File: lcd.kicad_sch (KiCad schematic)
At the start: 4 parts, among them J5 LS013B7DH03

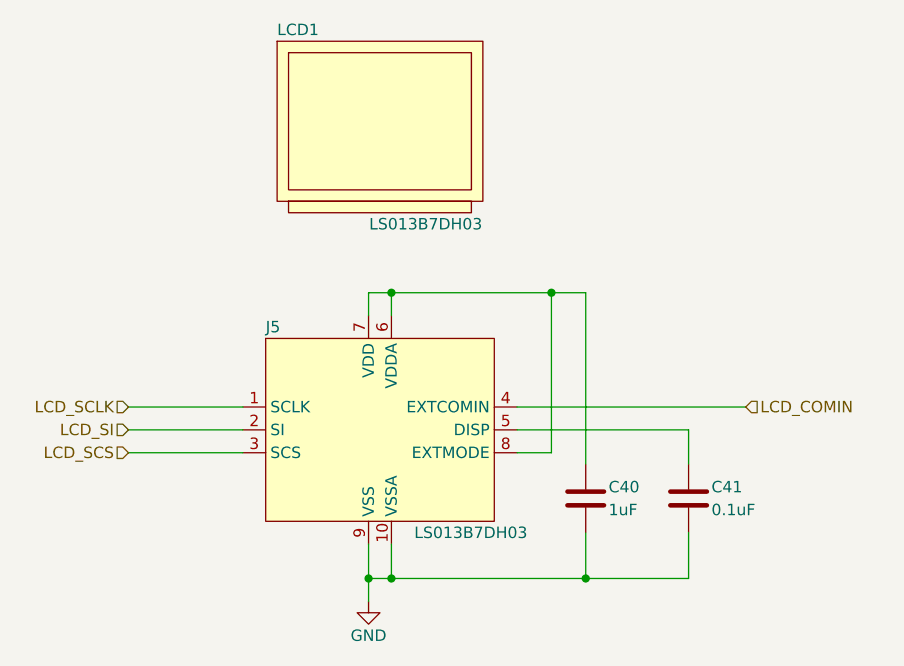
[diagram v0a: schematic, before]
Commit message: schematic cleanup
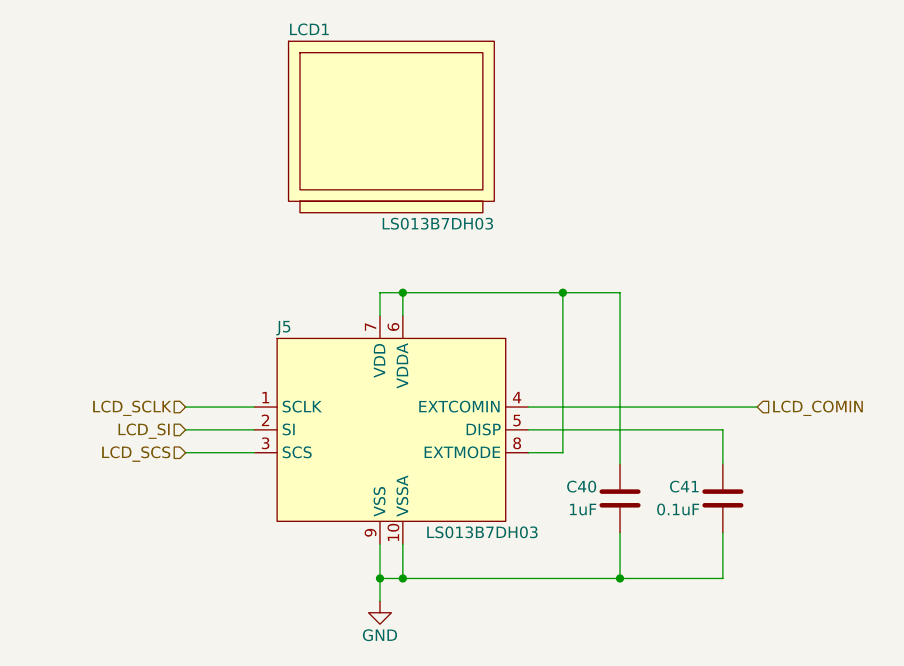
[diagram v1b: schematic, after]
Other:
- moved on the sheet: C40, C41, J5, LCD1
